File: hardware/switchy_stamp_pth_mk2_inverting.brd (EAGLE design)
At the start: 38.1 x 25.4 mm, 23 parts, among them IC1 MC34063

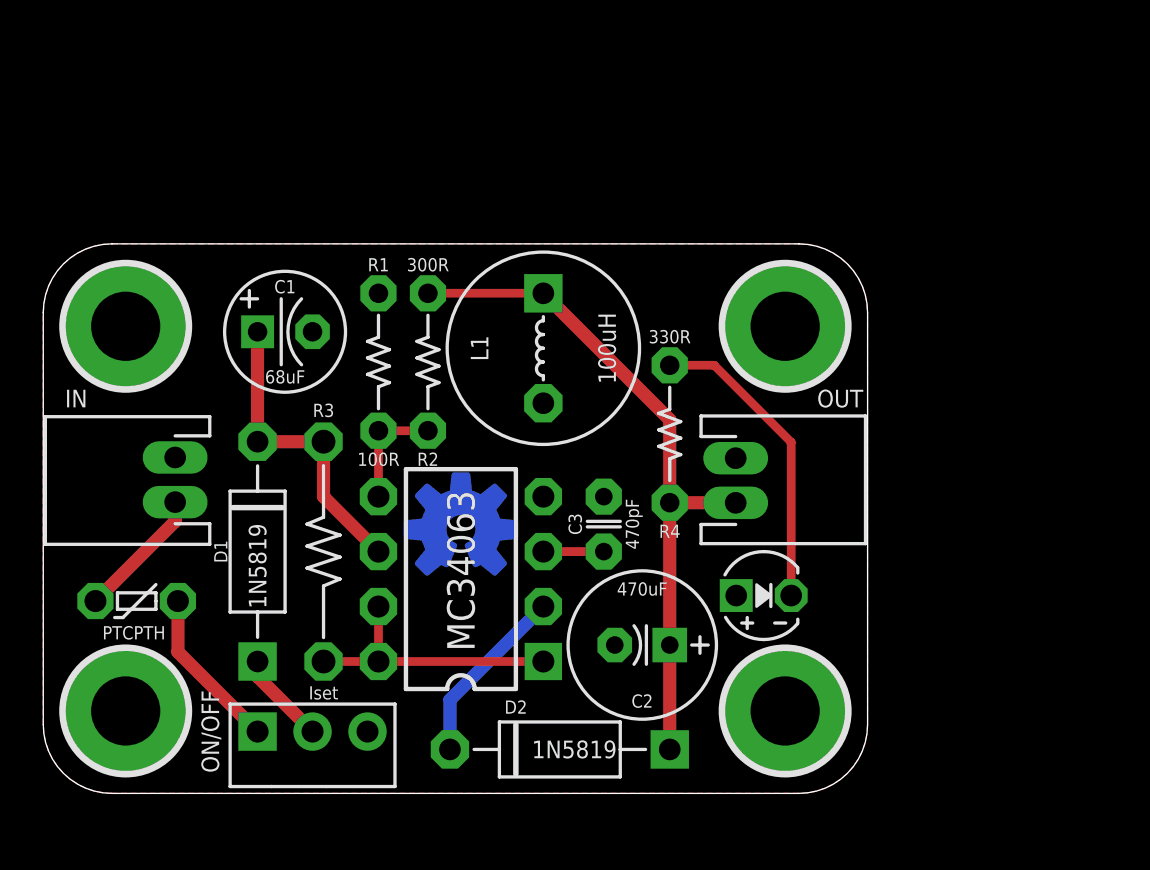
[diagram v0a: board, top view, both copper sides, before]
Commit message: fixed a few mistakes, still rearranging
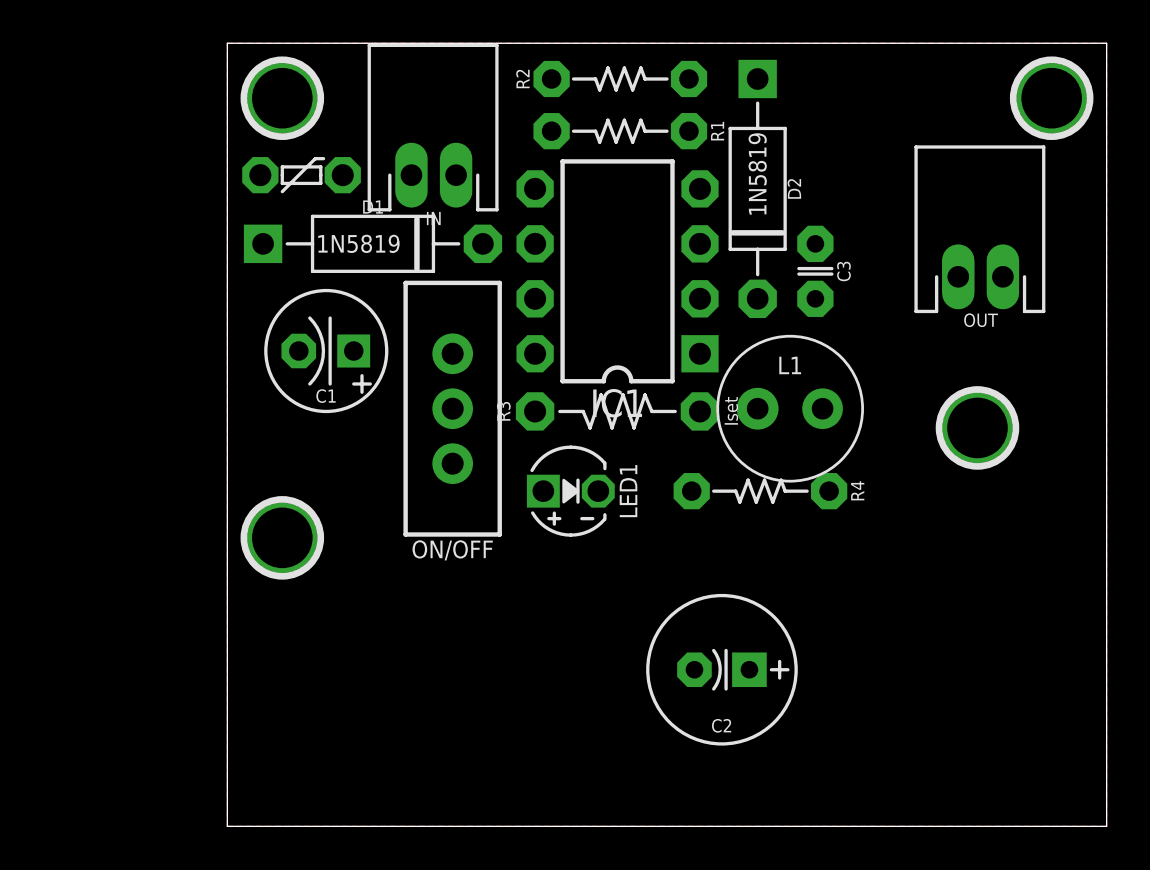
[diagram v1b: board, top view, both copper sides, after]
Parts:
- removed U$1: (no value), A_butts:CC-BY-SA-4.0-NO-URL
- removed U$2: (no value), A_butts:COW_SMALL
- removed U$3: (no value), A_butts:OSHWLOGO_BOT_0.2_A
- C1: value 68uF -> 100uF
- H1, H2, H3, H4: value HOLE#4 -> HOLE#2; device A_butts:HOLE-#4 -> A_butts:HOLE-#2
- L1: device A_butts:RLB0912 -> A_butts:RADIAL-PTH-3-BY-6.7DIA
- ON/OFF: value SWITCH-SPDTPTH-RA-2.54MM -> SWITCH-SPDTPTH-VERT-2.54MM; device A_butts:SPDT-RA-2.54MM -> A_butts:SWITCH-SPDT
- R3: device A_butts:RESISTOR-AXIAL-PTH-10.16MM -> A_butts:RESISTOR-AXIAL-PTH-7.68MM
- moved H4 51.3 mm to (46.6, 32.1)
- moved D2 27.5 mm to (33.0, 27.9), turned to 270 degrees
- moved H1 25.2 mm to (11.0, 11.8)
- moved F1 21.1 mm to (11.9, 28.6), turned to 0 degrees
- moved IN 18.6 mm to (17.0, 28.6), turned to 0 degrees
- moved ON/OFF 17.4 mm to (18.9, 17.8)
- moved IC1 16.0 mm to (26.5, 24.1)
- moved R2 15.8 mm to (26.7, 33.0), turned to 0 degrees
- moved H3 15.8 mm to (43.2, 16.9)
- moved R1 15.5 mm to (26.7, 30.6), turned to 180 degrees
- moved C3 15.2 mm to (35.7, 24.1), turned to 270 degrees
- moved D1 15.2 mm to (15.2, 25.4), turned to 0 degrees
- moved R3 15.1 mm to (26.5, 17.7), turned to 0 degrees
- moved OUT 13.3 mm to (42.3, 23.9), turned to 0 degrees
- moved H2 12.8 mm to (11.0, 32.1)
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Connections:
- net GND: now also L1.P$2; no longer L1.2
- net N$6: now also L1.P$1
- net VOUT-: no longer L1.1
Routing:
- net VOUT-: track 31.9 -> 0.00 mm
- net N$5: track 14.3 -> 0.00 mm
- net N$7: track 14.2 -> 0.00 mm
- net N$1: track 12.7 -> 0.00 mm
- net N$6: track 8.39 -> 0.00 mm
- net N$8: track 7.56 -> 0.00 mm
- net VIN+: track 6.10 -> 0.00 mm
- net N$3: track 5.33 -> 0.00 mm
- net N$4: track 4.29 -> 0.00 mm
- net N$2: track 2.79 -> 0.00 mm
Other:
- board size 38.1 x 25.4 mm -> 40.6 x 36.2 mm

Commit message: redo
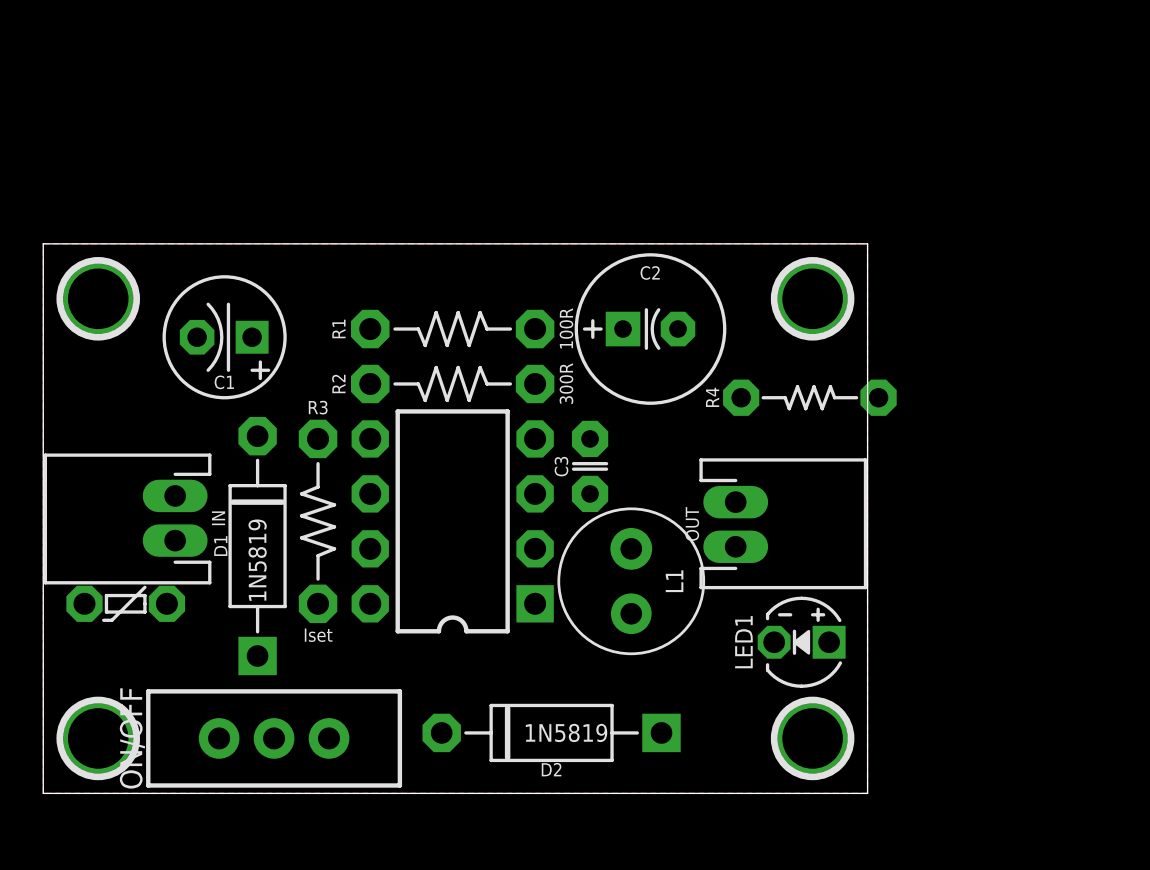
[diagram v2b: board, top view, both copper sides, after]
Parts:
- R1, R2: device A_butts:RESISTOR-AXIAL-PTH-5.08MM -> A_butts:RESISTOR-AXIAL-PTH-7.68MM
- moved H4 31.6 mm to (35.6, 2.54)
- moved D2 26.9 mm to (23.5, 2.79), turned to 180 degrees
- moved F1 21.4 mm to (3.81, 8.76), turned to 180 degrees
- moved IN 20.1 mm to (6.10, 11.7), turned to 90 degrees
- moved ON/OFF 17.3 mm to (10.7, 2.54), turned to 90 degrees
- moved C2 16.1 mm to (28.1, 21.5), turned to 0 degrees
- moved R2 16.1 mm to (18.9, 18.9)
- moved D1 15.0 mm to (9.91, 11.4), turned to 90 degrees
- moved R3 14.7 mm to (12.7, 12.6), turned to 270 degrees
- moved OUT 14.6 mm to (32.0, 13.5), turned to 270 degrees
- moved IC1 13.8 mm to (18.9, 12.6)
- moved C3 13.8 mm to (25.3, 15.1), turned to 90 degrees
- moved LED1 12.8 mm to (35.1, 6.99), turned to 180 degrees
- moved H1 12.6 mm to (2.54, 2.54)
- moved H2 12.6 mm to (2.54, 22.9)
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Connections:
- net N$4: now also F1.P$1; no longer ON/OFF.2
- net N$8: now also F1.P$2, ON/OFF.2; no longer F1.P$1, ON/OFF.1
- net VIN+: now also ON/OFF.3; no longer F1.P$2
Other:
- board size 40.6 x 36.2 mm -> 38.1 x 25.4 mm
